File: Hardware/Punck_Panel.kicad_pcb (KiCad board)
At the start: 2 copper layers, 91.2 x 128.5 mm, 41 parts

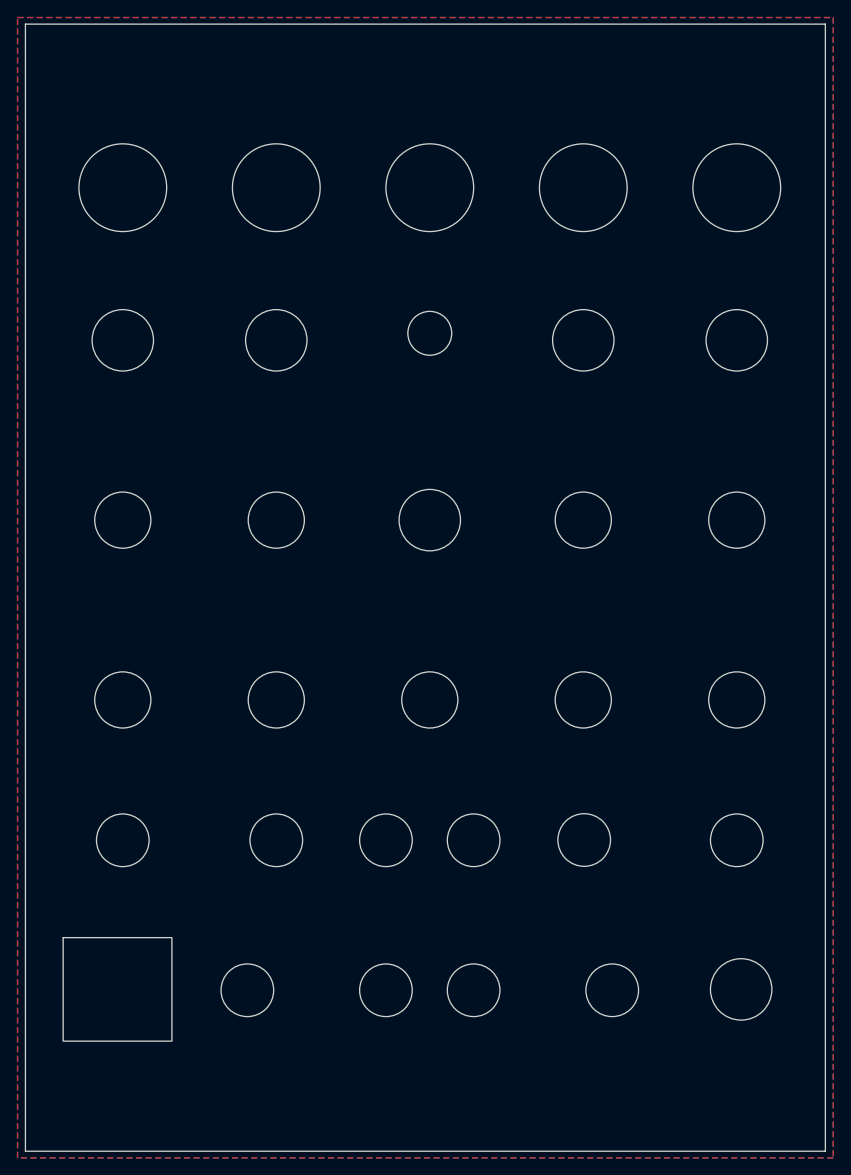
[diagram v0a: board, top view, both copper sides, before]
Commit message: Final tweaking and v1 gerber creation; JLC order placed
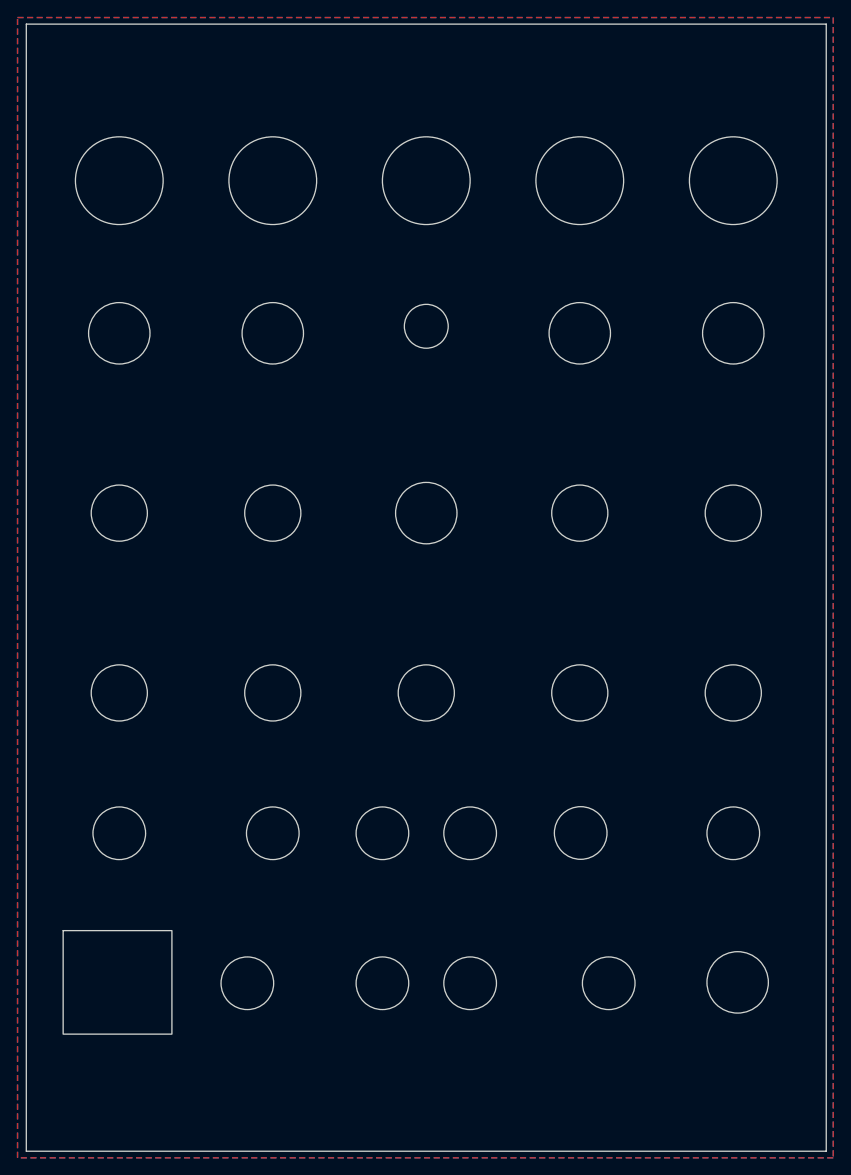
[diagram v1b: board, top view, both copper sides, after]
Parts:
- moved Ref** 0.89 mm to (133.2, 133.0)
- moved Ref** 0.89 mm to (120.6, 150.1)
- moved Ref** 0.89 mm to (136.4, 150.1)
- moved Ref** 0.89 mm to (98.1, 133.0)
- moved Ref** 0.89 mm to (110.6, 150.1)
- moved Ref** 0.89 mm to (80.6, 133.0)
- moved Ref** 0.89 mm to (151.1, 150.0)
- moved Ref** 0.89 mm to (120.6, 133.0)
- moved Ref** 0.89 mm to (150.6, 133.0)
- moved Ref** 0.89 mm to (110.6, 133.0)
- moved G*** 0.89 mm to (115.6, 43.9)
- moved Ref** 0.89 mm to (133.1, 96.5)
- moved Ref** 0.89 mm to (98.1, 117.0)
- moved Ref** 0.89 mm to (133.1, 117.0)
- moved Ref** 0.89 mm to (80.6, 58.6)
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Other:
- board text added: "JLCJLCJLCJLC"
- board text added: "Mountjoy Modular Punck Panel v1.0"
